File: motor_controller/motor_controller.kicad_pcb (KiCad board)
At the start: 4 copper layers, 98 x 98 mm, 182 parts, among them J1 Conn_01x03, J2 Conn_01x02, J3 Conn_01x03, J4 Conn_01x03, J5 Conn_01x03, J6 uart, J7 etm, J8 encoder, U1 INA186A3IYFDR, U3 STM32G474VEHx

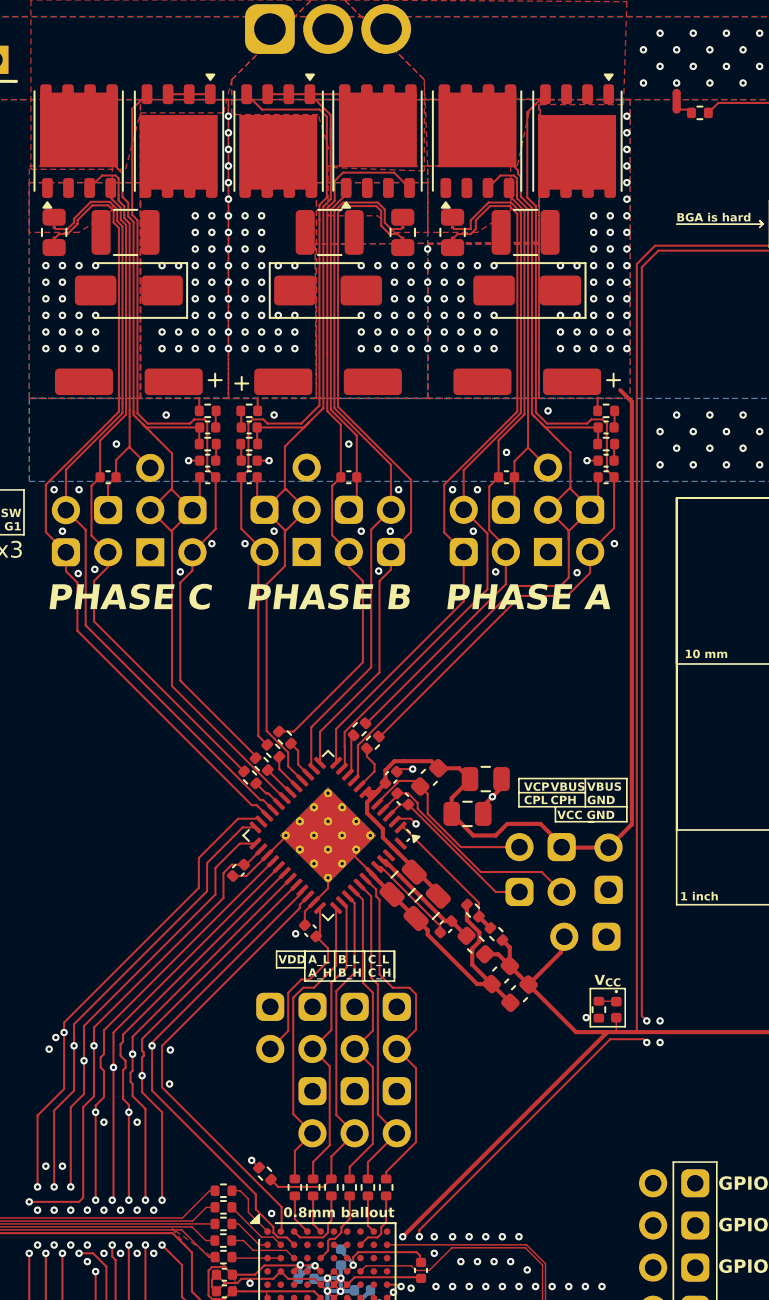
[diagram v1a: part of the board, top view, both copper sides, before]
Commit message: e
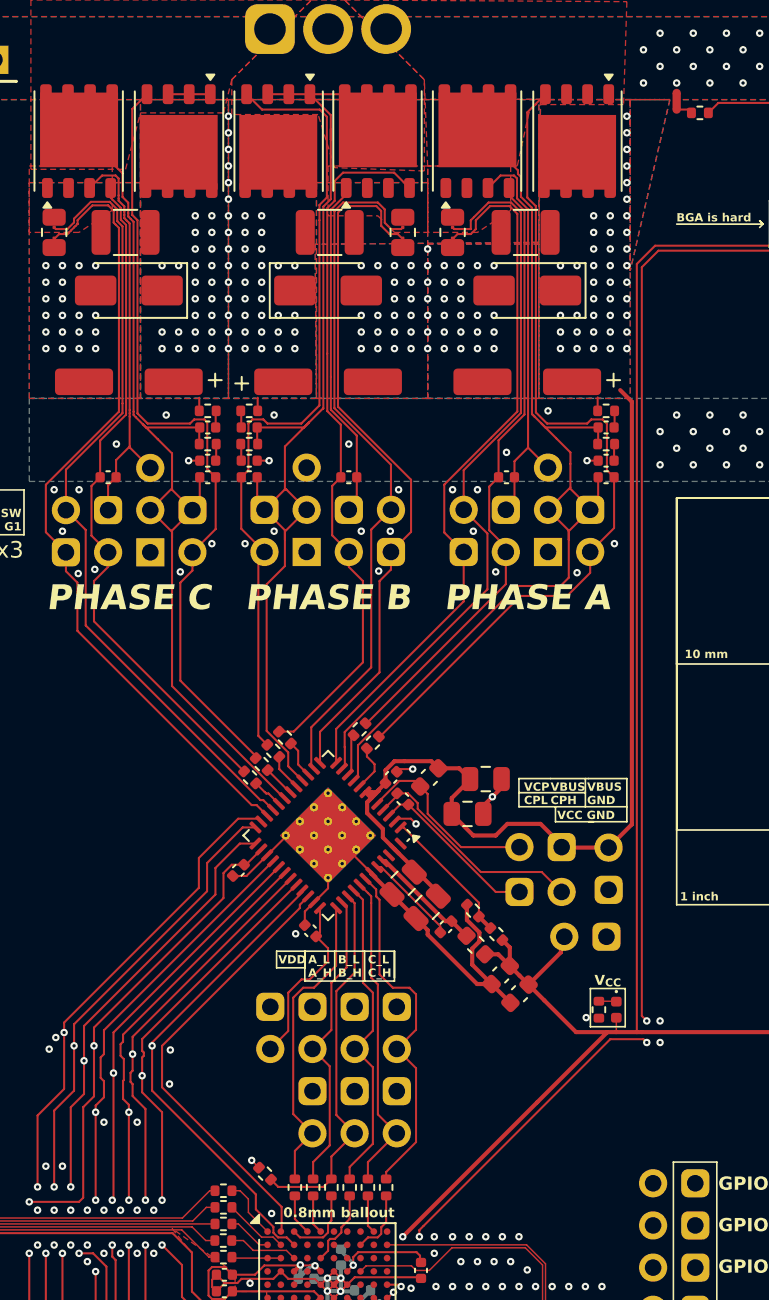
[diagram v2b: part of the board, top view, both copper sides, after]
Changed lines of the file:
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@@
 	)
 	(segment
-		(start 55.5 96.1)
-		(end 55.5 94.5)
+		(start 63.2 113.4)
+		(end 64.084901 112.515099)
 		(width 0.125)
 		(layer "F.Cu")
@@
 	)
 	(segment
-		(start 63.2 113.4)
-		(end 64.084901 112.515099)
+		(start 55.5 95.13)
+		(end 55.3 94.93)
 		(width 0.125)
 		(layer "F.Cu")
@@
 	)
 	(segment
-		(start 55.5 94.5)
-		(end 55.3 94.3)
+		(start 55 97)
+		(end 55 96.6)
 		(width 0.125)
 		(layer "F.Cu")
@@
 	)
 	(segment
-		(start 66.155584 111.674416)
-		(end 65.314901 112.515099)
+		(start 55.3 94.93)
+		(end 55.3 93.7)
 		(width 0.125)
 		(layer "F.Cu")
@@
 	)
 	(segment
-		(start 55.3 94.3)
-		(end 55.3 93.7)
+		(start 66.155584 111.674416)
+		(end 65.314901 112.515099)
 		(width 0.125)
 		(layer "F.Cu")
@@
 	)
 	(segment
-		(start 55 97)
-		(end 55 102.3)
+		(start 55.5 96.1)
+		(end 55.5 95.13)
 		(width 0.125)
 		(layer "F.Cu")
@@
 	)
 	(segment
-		(start 55.3 93.7)
-		(end 55.5 93.5)
+		(start 55.5 92.062232)
+		(end 65.685437 81.876796)
 		(width 0.125)
 		(layer "F.Cu")
@@
 	)
 	(segment
-		(start 64.314901 112.515099)
-		(end 64.296086 112.5151)
+		(start 55.3 93.7)
+		(end 55.5 93.5)
 		(width 0.125)
 		(layer "F.Cu")
@@
 	)
 	(segment
-		(start 66.155584 111.388729)
-		(end 66.155584 111.674416)
+		(start 55 96.6)
+		(end 55.5 96.1)
 		(width 0.125)
 		(layer "F.Cu")
@@
 	)
 	(segment
-		(start 55.5 93.5)
-		(end 55.5 92.062232)
+		(start 55 97)
+		(end 55 102.3)
 		(width 0.125)
 		(layer "F.Cu")
@@
 	)
 	(segment
-		(start 55 96.6)
-		(end 55.5 96.1)
+		(start 64.314901 112.515099)
+		(end 64.296086 112.5151)
 		(width 0.125)
 		(layer "F.Cu")
@@
 	)
 	(segment
-		(start 55.5 92.062232)
-		(end 65.685437 81.876796)
+		(start 66.155584 111.388729)
+		(end 66.155584 111.674416)
 		(width 0.125)
 		(layer "F.Cu")
@@
 	)
 	(segment
-		(start 55 97)
-		(end 55 96.6)
+		(start 55.5 93.5)
+		(end 55.5 92.062232)
 		(width 0.125)
 		(layer "F.Cu")
@@
 	)
 	(segment
-		(start 56.8 94.325003)
-		(end 56.8 93.9)
-		(width 0.125)
-		(layer "F.Cu")
-		(net "/DRV_MOSI")
-	)
-	(segment
 		(start 56.650006 92.749994)
 		(end 56.650006 92.326441)
@@
 	)
 	(segment
-		(start 57 96.55)
-		(end 56.650006 96.200006)
+		(start 56.7 93.8)
+		(end 56.5 93.6)
 		(width 0.125)
 		(layer "F.Cu")
@@
 	)
 	(segment
-		(start 56.5 93.6)
-		(end 56.5 92.9)
+		(start 56.650006 96.200006)
+		(end 56.650006 95.109994)
 		(width 0.125)
 		(layer "F.Cu")
@@
 	)
 	(segment
-		(start 56.650006 94.474997)
-		(end 56.8 94.325003)
+		(start 56.5 93.6)
+		(end 56.5 92.9)
 		(width 0.125)
 		(layer "F.Cu")
@@
 	)
 	(segment
-		(start 56.650006 96.200006)
-		(end 56.650006 94.474997)
+		(start 57 96.55)
+		(end 56.650006 96.200006)
 		(width 0.125)
 		(layer "F.Cu")
@@
 	)
 	(segment
-		(start 56.8 93.9)
-		(end 56.5 93.6)
+		(start 58.63 111.13)
+		(end 62.290001 111.13)
 		(width 0.125)
 		(layer "F.Cu")
@@
 	)
 	(segment
-		(start 56.5 92.9)
-		(end 56.650006 92.749994)
+		(start 56.7 95.06)
+		(end 56.7 93.8)
 		(width 0.125)
 		(layer "F.Cu")
@@
 	)
 	(segment
-		(start 58.63 111.13)
-		(end 62.290001 111.13)
+		(start 56.650006 92.326441)
+		(end 66.392544 82.583903)
 		(width 0.125)
 		(layer "F.Cu")
@@
 	)
 	(segment
-		(start 56.650006 92.326441)
-		(end 66.392544 82.583903)
+		(start 56.650006 95.109994)
+		(end 56.7 95.06)
 		(width 0.125)
 		(layer "F.Cu")
@@
 	)
 	(segment
+		(start 56.5 92.9)
+		(end 56.650006 92.749994)
+		(width 0.125)
+		(layer "F.Cu")
+		(net "/DRV_MOSI")
+	)
+	(segment
 		(start 57 109.5)
 		(end 58.63 111.13)
@@
 	)
 	(segment
-		(start 56.075003 92.194336)
-		(end 66.03899 82.230349)
+		(start 43.18 86.36)
+		(end 42.1776 85.3576)
 		(width 0.125)
 		(layer "F.Cu")
@@
 	)
 	(segment
-		(start 43.18 86.36)
-		(end 42.1776 85.3576)
+		(start 56.075003 102.224997)
+		(end 56 102.3)
+		(width 0.125)
+		(layer "F.Cu")
+		(net "/DRV_MISO")
+	)
+	(segment
+		(start 56.075003 92.194336)
+		(end 66.03899 82.230349)
 		(width 0.125)
 		(layer "F.Cu")
@@
 	)
 	(segment
-		(start 56.2 109.6)
-		(end 58.73 112.13)
-		(width 0.125)
-		(layer "F.Cu")
-		(net "/DRV_MISO")
-	)
-	(segment
-		(start 56.075003 102.224997)
-		(end 56 102.3)
+		(start 56.075003 94.64)
+		(end 56.075003 102.224997)
 		(width 0.125)
 		(layer "F.Cu")
@@
 	)
 	(segment
-		(start 56.075003 94.3)
-		(end 56.075003 102.224997)
+		(start 56.075003 94.64)
+		(end 56.075003 92.194336)
 		(width 0.125)
 		(layer "F.Cu")
@@
 	)
 	(segment
-		(start 56.075003 94.3)
-		(end 56.075003 92.194336)
+		(start 56.2 109.6)
+		(end 58.73 112.13)
 		(width 0.125)
 		(layer "F.Cu")
@@
 	)
 	(via
-		(at 56.075003 94.3)
+		(at 56.075003 94.64)
 		(size 0.45)
 		(drill 0.2)
@@
 	)
 	(segment
-		(start 56 105)
-		(end 56 102.3)
+		(start 56.075003 94.64)
+		(end 56.075003 92.990225)
 		(width 0.125)
 		(layer "In2.Cu")
@@
 	)
 	(segment
-		(start 56.075003 94.3)
-		(end 56.075003 92.990225)
+		(start 56 105)
+		(end 56 102.3)
 		(width 0.125)
 		(layer "In2.Cu")
@@
 	)
 	(segment
-		(start 49.444778 86.36)
-		(end 43.18 86.36)
+		(start 56.075003 92.990225)
+		(end 49.444778 86.36)
 		(width 0.125)
 		(layer "In2.Cu")
@@
 	)
 	(segment
-		(start 56.075003 92.990225)
-		(end 49.444778 86.36)
+		(start 49.444778 86.36)
+		(end 43.18 86.36)
 		(width 0.125)
 		(layer "In2.Cu")
@@
 			)
 		)
+	)
+	(zone
+		(net "VBUS")
+		(layers "F.Cu" "B.Cu" "In1.Cu" "In2.Cu")
+		(hatch edge 0.5)
+		(priority 10)
+		(connect_pads yes
+			(clearance 0)
+		)
+		(min_thickness 0.25)
+		(fill yes
+			(thermal_gap 0.5)
+			(thermal_bridge_width 0.5)
+			(island_removal_mode 0)
+		)
+		(polygon
+			(pts
+				(xy 89.59 36) (xy 87.2 46.31) (xy 87.2 36)
+			)
+		)
